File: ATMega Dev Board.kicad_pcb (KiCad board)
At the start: 4 copper layers, 84 x 38.1 mm, 50 parts, among them J1 Conn_01x13, J2 Conn_01x09, J4 SPI header, J5 USB-C_31-M-12, Q1 S8050, Q2 2N7002, Q3 HL6042, Q4 HL6042, SW1 SW_SPST, SW2 SW_SPST, U1 ATmega32A-A, U2 CH340C, U3 USBLC6-2P6, X1 16MHz

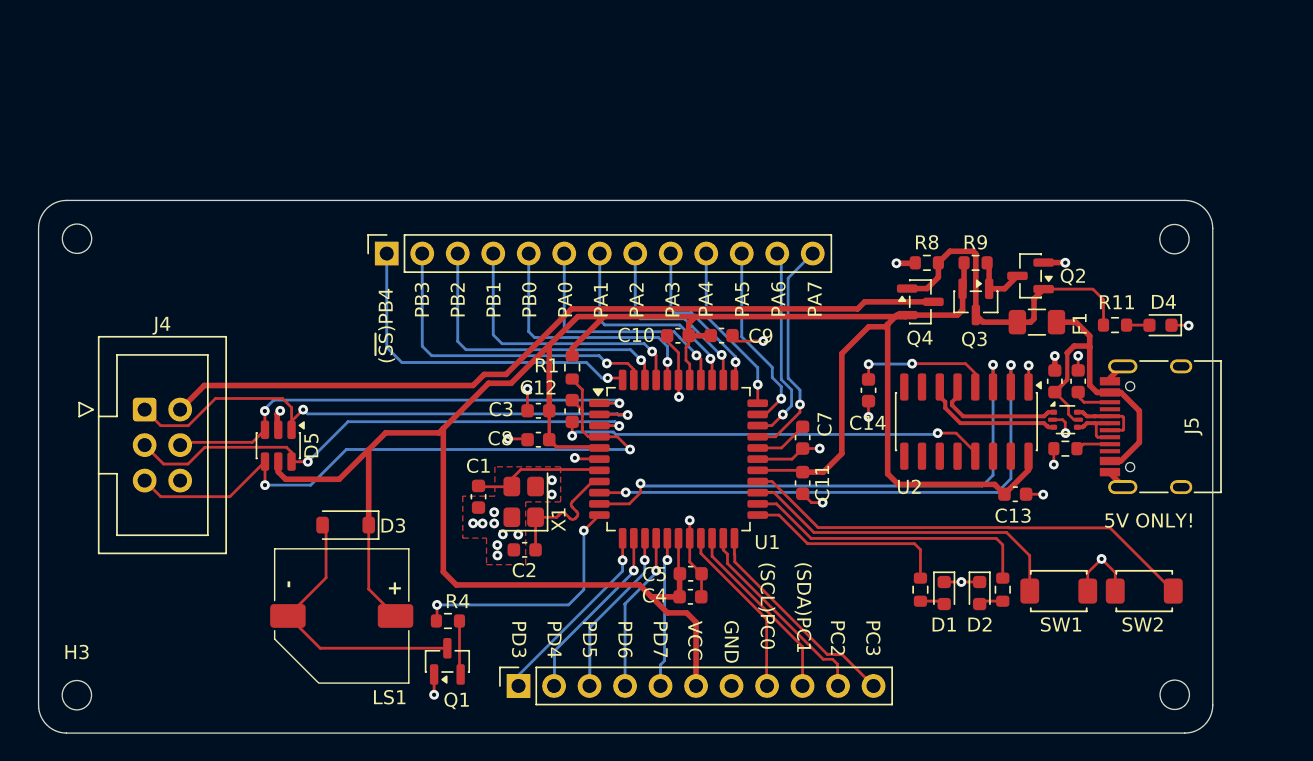
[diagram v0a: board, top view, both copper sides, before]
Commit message: Rev B layout
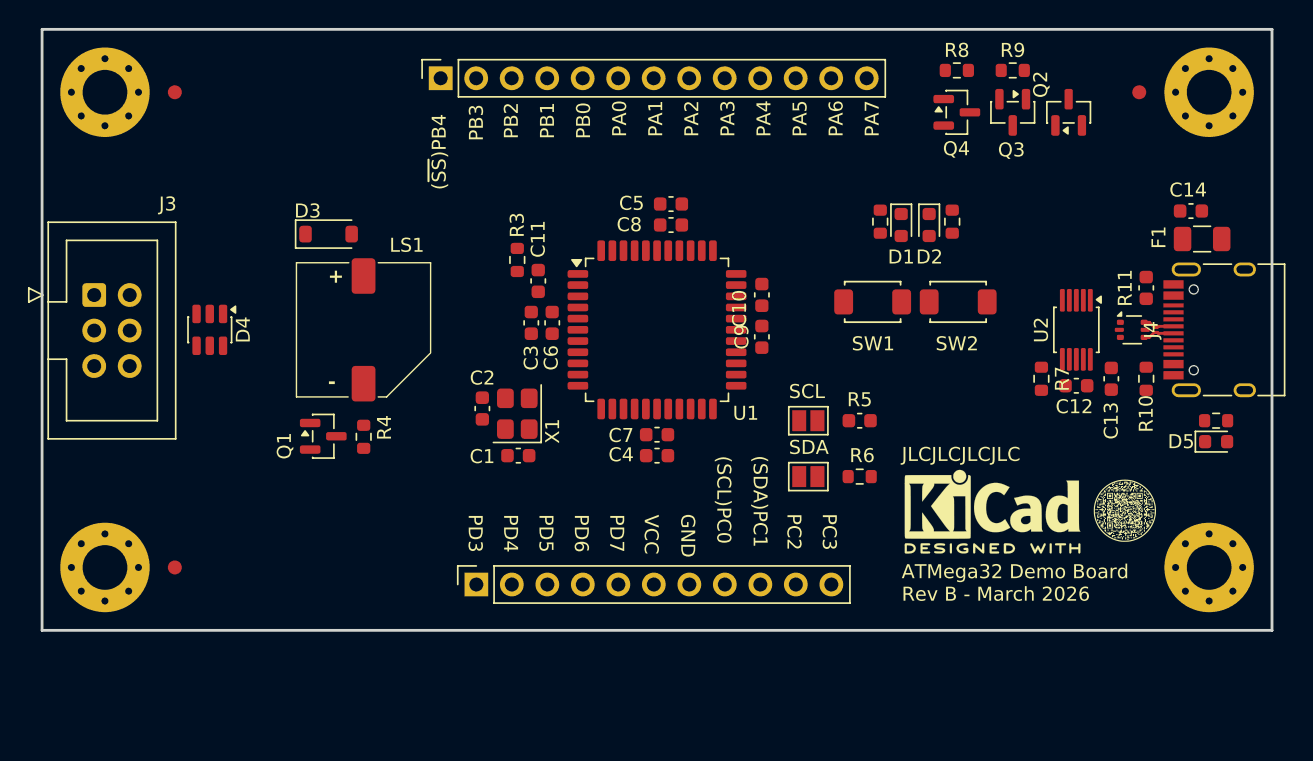
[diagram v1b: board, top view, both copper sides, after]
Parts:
- removed the G*** at (70.3, 71.7)
- added FID1: Fiducial, Fiducial:Fiducial_1mm_Mask2mm, F.Cu at (47.6, 48.4)
- added FID2: Fiducial, Fiducial:Fiducial_1mm_Mask2mm, F.Cu at (47.6, 82.4)
- added FID3: Fiducial, Fiducial:Fiducial_1mm_Mask2mm, F.Cu at (116.6, 48.4)
- added G***: LOGO, ATMDBL:qrcode, F.Cu at (115.6, 78.4)
- added JP1: Jumper_2_Small_Open, Jumper:SolderJumper-2_P1.3mm_Open_Pad1.0x1.5mm, F.Cu at (92.9, 71.9)
- added JP2: Jumper_2_Small_Open, Jumper:SolderJumper-2_P1.3mm_Open_Pad1.0x1.5mm, F.Cu at (92.9, 75.9)
- added R5: 5k1, Capacitor_SMD:C_0603_1608Metric, F.Cu at (96.6, 71.9)
- added R6: 5k1, Resistor_SMD:R_0603_1608Metric, F.Cu at (96.6, 75.9)
- added R7: 4k7, Resistor_SMD:R_0603_1608Metric, F.Cu at (109.6, 68.9)
- H1, H2, H3, H4: footprint MountingHole:MountingHole_2.1mm -> MountingHole:MountingHole_3.2mm_M3_Pad_Via
- J4: renamed from J5; footprint FTBLib:USB_C_Receptacle_HRO_TYPE-C-31-M-12 -> ATMDBL:USB_C_Receptacle_HRO_TYPE-C-31-M-12
- LS1: footprint FTBLib:Buzzer_MLT-9650 -> ATMDBL:Buzzer_MLT-9650
- REF**: moved to F.Cu
- SW1, SW2: footprint FTBLib:Switch_TS-1088-AR02016 -> ATMDBL:Switch_TS-1088-AR02016
- U2: footprint Package_SO:SOIC-16_3.9x9.9mm_P1.27mm -> Package_SO:MSOP-10_3x3mm_P0.5mm
- moved R2 26.6 mm to (103.2, 57.6)
- moved D2 26.6 mm to (101.5, 57.9)
- moved D1 26.5 mm to (99.5, 57.9)
- moved R1 26.5 mm to (98.0, 57.6)
- moved SW1 24.6 mm to (97.5, 63.4)
- moved SW2 24.6 mm to (103.6, 63.4)
- moved D3 20.9 mm to (58.6, 58.5), turned to 0 degrees
- moved LS1 20.5 mm to (61.1, 65.4), turned to 0 degrees
- moved Q1 18.4 mm to (58.2, 73.0), turned to 0 degrees
- moved C13 17.4 mm to (114.6, 68.9)
- moved REF** 16.3 mm to (106.1, 78.4), turned to 0 degrees
- moved C14 15.6 mm to (120.3, 56.9), turned to 180 degrees
- moved R4 14.5 mm to (61.1, 73.0), turned to 90 degrees
- moved R9 14.0 mm to (107.5, 46.8)
- moved R8 13.9 mm to (103.5, 46.8)
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- renumbered C2 to C1, C7 to C10, C12 to C11, C13 to C12, C14 to C13, C6 to C14, C1 to C2, C9 to C5, C8 to C6, C5 to C7, C10 to C8, C11 to C9, D5 to D4, D4 to D5, J4 to J3, R2 to R1, R5 to R10, R6 to R11, R11 to R12, R3 to R2, R1 to R3
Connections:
- net /PC0 renamed /SCL
- net /PC1 renamed /SDA
- C11 pad 2: Net-(U2-~{DTR}) -> /DTR
- C13 pad 2: Net-(U2-V3) -> /V3
- C14 pad 1: VBUS -> VUSB
- R12 pad 1: VUSB -> VBUS
- U1 pad 25: /SW1 -> /SW2
- U1 pad 26: /SW2 -> /SW1
- U2 pad 1: GND -> /UD+
- U2 pad 10: unconnected-(U2-~{DSR}-Pad10) -> /V3
- U2 pad 2: /UTXD -> /UD-
- U2 pad 3: /URXD -> GND
- U2 pad 4: Net-(U2-V3) -> unconnected-(U2-~{RTS}-Pad4)
- U2 pad 5: /UD+ -> unconnected-(U2-~{CTS}-Pad5)
- U2 pad 6: /UD- -> /DTR
- U2 pad 7: unconnected-(U2-NC-Pad7) -> VCC
- U2 pad 8: unconnected-(U2-NC-Pad8) -> /UTXD
- U2 pad 9: unconnected-(U2-~{CTS}-Pad9) -> /URXD
- U3 pad 1: /UD+ -> /UD-
- U3 pad 3: /UD- -> /UD+
- U3 pad 4: /UD_N -> /UD_P
- U3 pad 6: /UD_P -> /UD_N
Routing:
- net VCC: track 175.3 -> 0.00 mm
- net VSPI: track 57.1 -> 0.00 mm
- net GND: track 50.4 -> 0.00 mm, vias 32 -> 0
- net /RST: track 48.0 -> 0.00 mm, vias 2 -> 0
- net /MISO: track 40.8 -> 0.00 mm, vias 2 -> 0
- net /UTXD: track 39.5 -> 0.00 mm, vias 2 -> 0
- net /URXD: track 39.0 -> 0.00 mm, vias 2 -> 0
- net /SCK: track 38.6 -> 0.00 mm, vias 2 -> 0
- net /MOSI: track 35.2 -> 0.00 mm, vias 2 -> 0
- net /SW2: track 33.0 -> 0.00 mm
- net Net-(U2-~{DTR}): track 30.9 -> 0.00 mm, vias 2 -> 0
- net /PB4: track 24.6 -> 0.00 mm, vias 1 -> 0
- net VUSB: track 24.4 -> 0.00 mm
- net /SW1: track 23.9 -> 0.00 mm
- net VBUS: track 23.4 -> 0.00 mm
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- removed copper zone on F.Cu, net GND
- removed copper zone on In1.Cu, net GND
- removed copper zone on In2.Cu, net GND
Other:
- board size 84 x 38.1 mm -> 88 x 43 mm
- board text added: "ATMega32 Demo Board Rev B - March 2026"
- board text added: "SCL"
- board text added: "SDA"
- board text removed: "5V ONLY!"
- board text removed: "ATMega32 Demo Board Rev A - March 2026 https://github.com/spassigl/ATMega32A-demo-board.git"
